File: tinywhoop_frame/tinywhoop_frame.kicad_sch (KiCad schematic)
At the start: 17 parts, among them J1 ESP_conn1, J2 ESP_conn2, J3 ESP_Unused_Pins1, J5 Batt_conn, J6 Conn_02x03_Counter_Clockwise, Q1 2N7002, Q2 2N7002, Q3 2N7002, Q4 2N7002

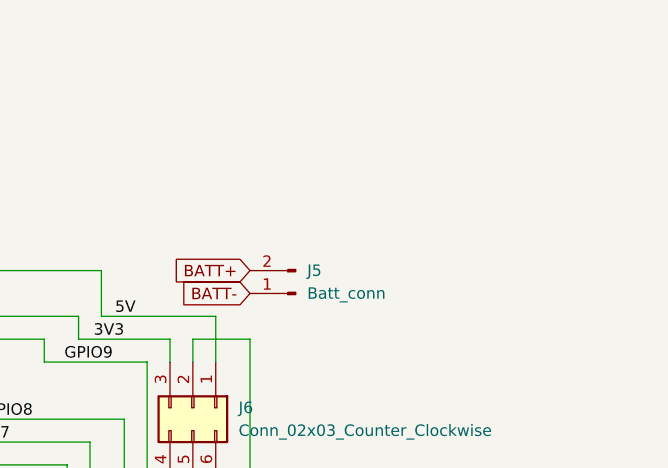
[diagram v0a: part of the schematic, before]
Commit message: pcb updates
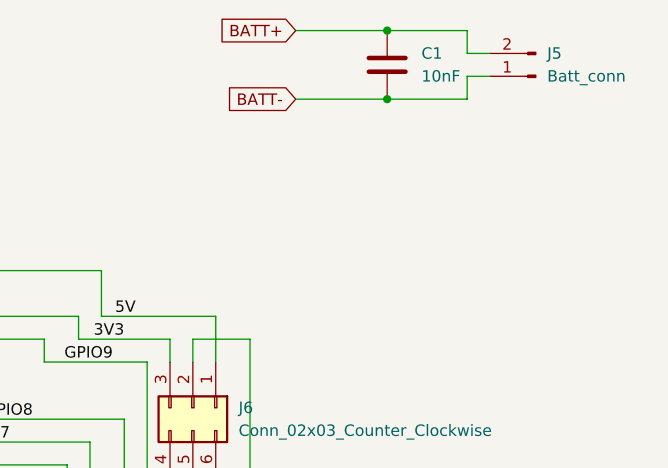
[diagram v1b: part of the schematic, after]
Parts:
- added C1: 10nF, Capacitor_SMD:C_0805_2012Metric_Pad1.18x1.45mm_HandSolder, symbol Device:C
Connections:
- net BATT+: now also C1.1
- net BATT-: now also C1.2
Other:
- moved on the sheet: J5
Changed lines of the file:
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@@
+	)
+	(junction
+		(at 241.3 21.59)
+		(diameter 0)
+		(color 0 0 0 0)
 	)
 	(junction
@@
 	)
 	(junction
+		(at 241.3 29.21)
+		(diameter 0)
+		(color 0 0 0 0)
+	)
+	(junction
 		(at 57.15 53.34)
 		(diameter 0)
@@
 	(wire
 		(pts
+			(xy 250.19 21.59) (xy 241.3 21.59)
+		)
+		(stroke
+			(width 0)
+			(type default)
+		)
+	)
+	(wire
+		(pts
 			(xy 171.45 67.31) (xy 173.99 67.31)
 		)
@@
 	(wire
 		(pts
+			(xy 250.19 26.67) (xy 252.73 26.67)
+		)
+		(stroke
+			(width 0)
+			(type default)
+		)
+	)
+	(wire
+		(pts
 			(xy 97.79 91.44) (xy 105.41 91.44)
 		)
@@
 	(wire
 		(pts
+			(xy 250.19 24.13) (xy 250.19 21.59)
+		)
+		(stroke
+			(width 0)
+			(type default)
+		)
+	)
+	(wire
+		(pts
 			(xy 57.15 96.52) (xy 62.23 96.52)
 		)
@@
 	(wire
 		(pts
+			(xy 231.14 29.21) (xy 241.3 29.21)
+		)
+		(stroke
+			(width 0)
+			(type default)
+		)
+	)
+	(wire
+		(pts
 			(xy 207.01 53.34) (xy 207.01 55.88)
 		)
@@
 	(wire
 		(pts
+			(xy 231.14 21.59) (xy 241.3 21.59)
+		)
+		(stroke
+			(width 0)
+			(type default)
+		)
+	)
+	(wire
+		(pts
 			(xy 219.71 73.66) (xy 219.71 71.12)
 		)
@@
 	(wire
 		(pts
+			(xy 252.73 24.13) (xy 250.19 24.13)
+		)
+		(stroke
+			(width 0)
+			(type default)
+		)
+	)
+	(wire
+		(pts
+			(xy 241.3 29.21) (xy 250.19 29.21)
+		)
+		(stroke
+			(width 0)
+			(type default)
+		)
+	)
+	(wire
+		(pts
 			(xy 187.96 63.5) (xy 187.96 69.85)
 		)
@@
 		(pts
 			(xy 168.91 63.5) (xy 168.91 69.85)
+		)
+		(stroke
+			(width 0)
+			(type default)
+		)
+	)
+	(wire
+		(pts
+			(xy 250.19 29.21) (xy 250.19 26.67)
 		)
 		(stroke
@@
 	(global_label "BATT-"
 		(shape input)
-		(at 226.06 50.8 180)
+		(at 231.14 29.21 180)
 		(fields_autoplaced yes)
 		(effects
@@
 		)
 		(property "Intersheetrefs" "${INTERSHEET_REFS}"
-			(at 217.2086 50.8 0)
+			(at 222.2886 29.21 0)
 			(effects
 				(font
@@
 	(global_label "BATT+"
 		(shape input)
-		(at 226.06 48.26 180)
+		(at 231.14 21.59 180)
 		(fields_autoplaced yes)
 		(effects
@@
 		)
 		(property "Intersheetrefs" "${INTERSHEET_REFS}"
-			(at 217.2086 48.26 0)
+			(at 222.2886 21.59 0)
 			(effects
 				(font
@@
 	(symbol
 		(lib_id "Connector:Conn_01x02_Pin")
-		(at 231.14 50.8 180)
+		(at 257.81 26.67 180)
 		(unit 1)
 		(exclude_from_sim no)
@@
 		(dnp no)
 		(property "Reference" "J5"
-			(at 232.41 48.2599 0)
+			(at 259.08 24.1299 0)
 			(effects
 				(font
@@
 		)
 		(property "Value" "Batt_conn"
-			(at 232.41 50.7999 0)
+			(at 259.08 26.6699 0)
 			(effects
 				(font
@@
 		)
 		(property "Footprint" "Connector_PinHeader_2.54mm:PinHeader_1x02_P2.54mm_Vertical"
-			(at 231.14 50.8 0)
+			(at 257.81 26.67 0)
 			(effects
 				(font
@@
 		)
 		(property "Datasheet" "~"
-			(at 231.14 50.8 0)
+			(at 257.81 26.67 0)
 			(effects
 				(font
@@
 		)
 		(property "Description" "Generic connector, single row, 01x02, script generated"
-			(at 231.14 50.8 0)
+			(at 257.81 26.67 0)
 			(effects
 				(font
@@
 					(unit 1)
 				)
+			)
+		)
+	)
+	(symbol
+		(lib_id "Device:C")
+		(at 241.3 25.4 0)
+		(unit 1)
+		(exclude_from_sim no)
+		(in_bom yes)
+		(on_board yes)
+		(dnp no)
+		(fields_autoplaced yes)
+		(property "Reference" "C1"
+			(at 245.11 24.1299 0)
+			(effects
+				(font
+					(size 1.27 1.27)
+				)
+				(justify left)
+			)
+		)
+		(property "Value" "10nF"
+			(at 245.11 26.6699 0)
+			(effects
+				(font
+					(size 1.27 1.27)
+				)
+				(justify left)
+			)
+		)
+		(property "Footprint" "Capacitor_SMD:C_0805_2012Metric_Pad1.18x1.45mm_HandSolder"
+			(at 242.2652 29.21 0)
+			(effects
+				(font
+					(size 1.27 1.27)
+				)
+				(hide yes)
+			)
+		)
+		(property "Datasheet" "~"
+			(at 241.3 25.4 0)
+			(effects
+				(font
+					(size 1.27 1.27)
+				)
+				(hide yes)
+			)
+		)
+		(property "Description" "Unpolarized capacitor"
+			(at 241.3 25.4 0)
+			(effects
+				(font
+					(size 1.27 1.27)
+				)
+				(hide yes)
+			)
+		)
+		(pin "1"
+		)
+		(pin "2"
+		)
+		(instances
+			(project ""
+				(path "/dcf85f80-a84f-42ea-b7be-95670bbb8f64"
+					(reference "C1")
+					(unit 1)
+				)

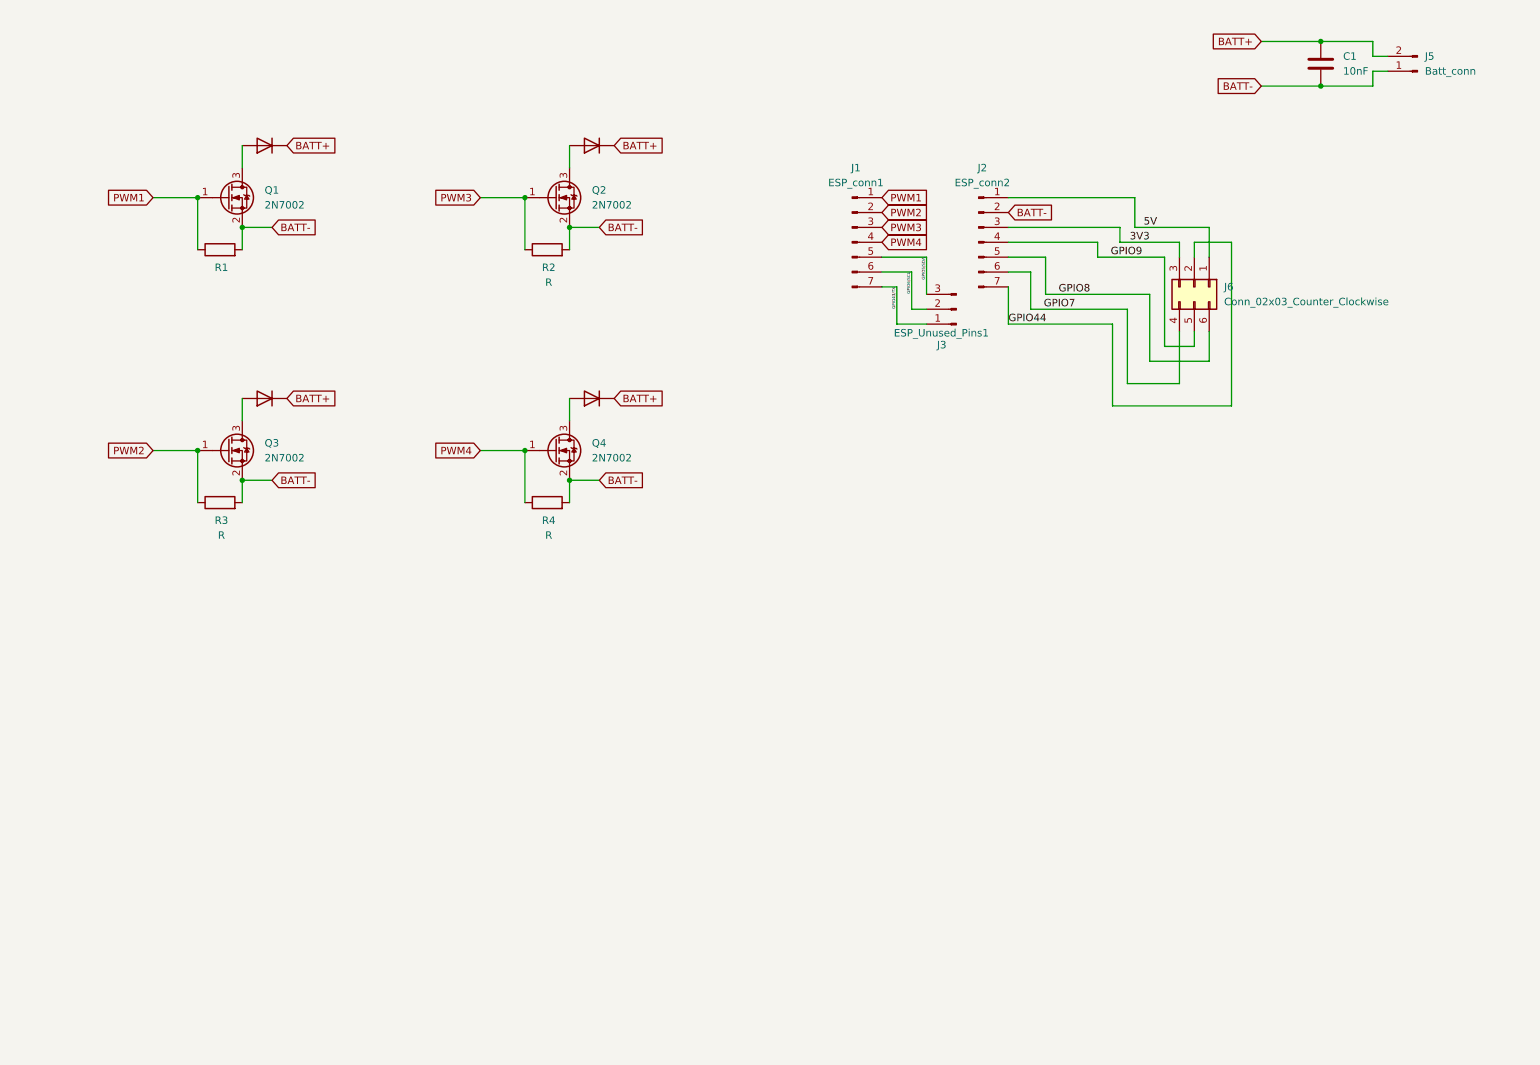
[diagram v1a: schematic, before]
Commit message: updated pcb
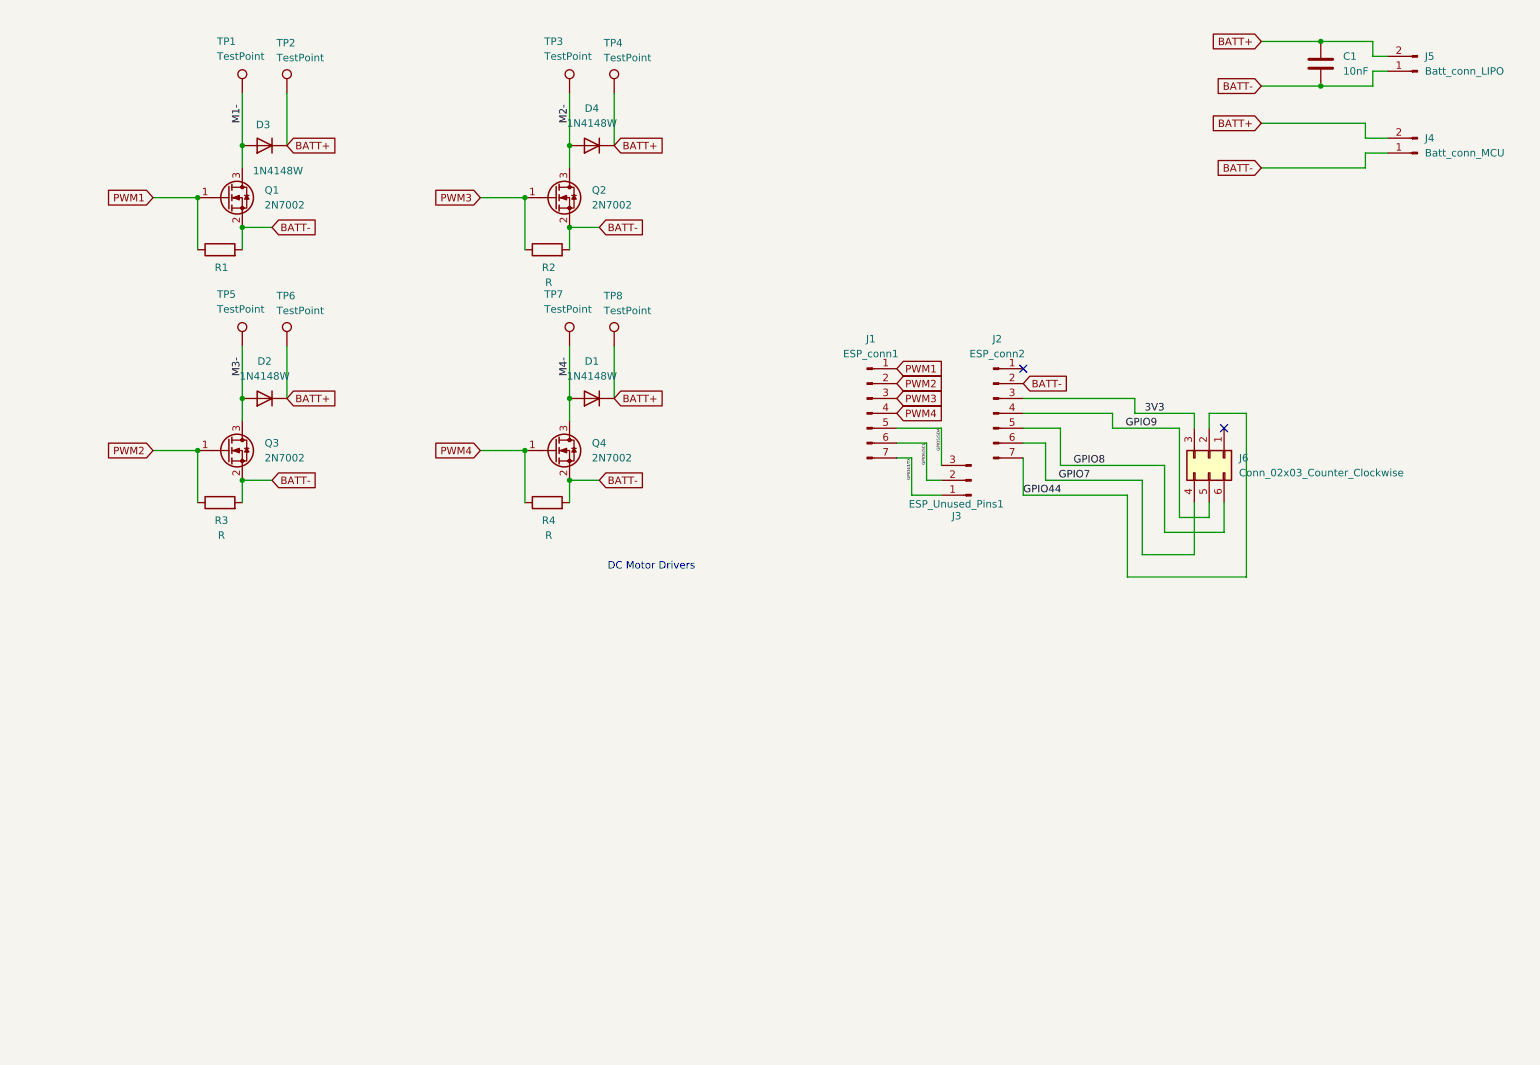
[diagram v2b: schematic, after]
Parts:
- removed D1, D2, D3, D4: D, Diode_THT:D_DO-35_SOD27_P7.62mm_Horizontal, symbol Device:D
- added D1, D2, D3, D4: 1N4148W, Diode_SMD:D_SOD-123, symbol Diode:1N4148W
- added J4: Batt_conn_MCU, Connector_PinHeader_2.54mm:PinHeader_1x02_P2.54mm_Vertical, symbol Connector:Conn_01x02_Pin
- added TP1, TP2, TP3, TP4, TP5, TP6, TP7, TP8: TestPoint, TestPoint:TestPoint_Pad_1.5x1.5mm, symbol Connector:TestPoint
- J5: value Batt_conn -> Batt_conn_LIPO
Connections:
- net BATT+: now also D1.1 (K), D2.1 (K), D3.1 (K), D4.1 (K), J4.2 (Pin_2), TP2.1, TP4.1, TP6.1, TP8.1
- net BATT-: now also J4.1 (Pin_1)
- net M4-: now reaches Q4.3 (D)
- net M4-: now also D1.2 (A), TP7.1
- net M3-: now reaches Q3.3 (D)
- net M3-: now also D2.2 (A), TP5.1
- net M1-: now reaches Q1.3 (D)
- net M1-: now also D3.2 (A), TP1.1
- net M2-: now reaches Q2.3 (D)
- net M2-: now also D4.2 (A), TP3.1
- net 5V: no longer names the net of J6.1 (Pin_1)
- net 5V: no longer J2.1 (Pin_1)
- no-connect marks 0 -> 2
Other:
- note added: "DC Motor Drivers"
- moved on the sheet: J1, J2, J3, J6

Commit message: pcb update
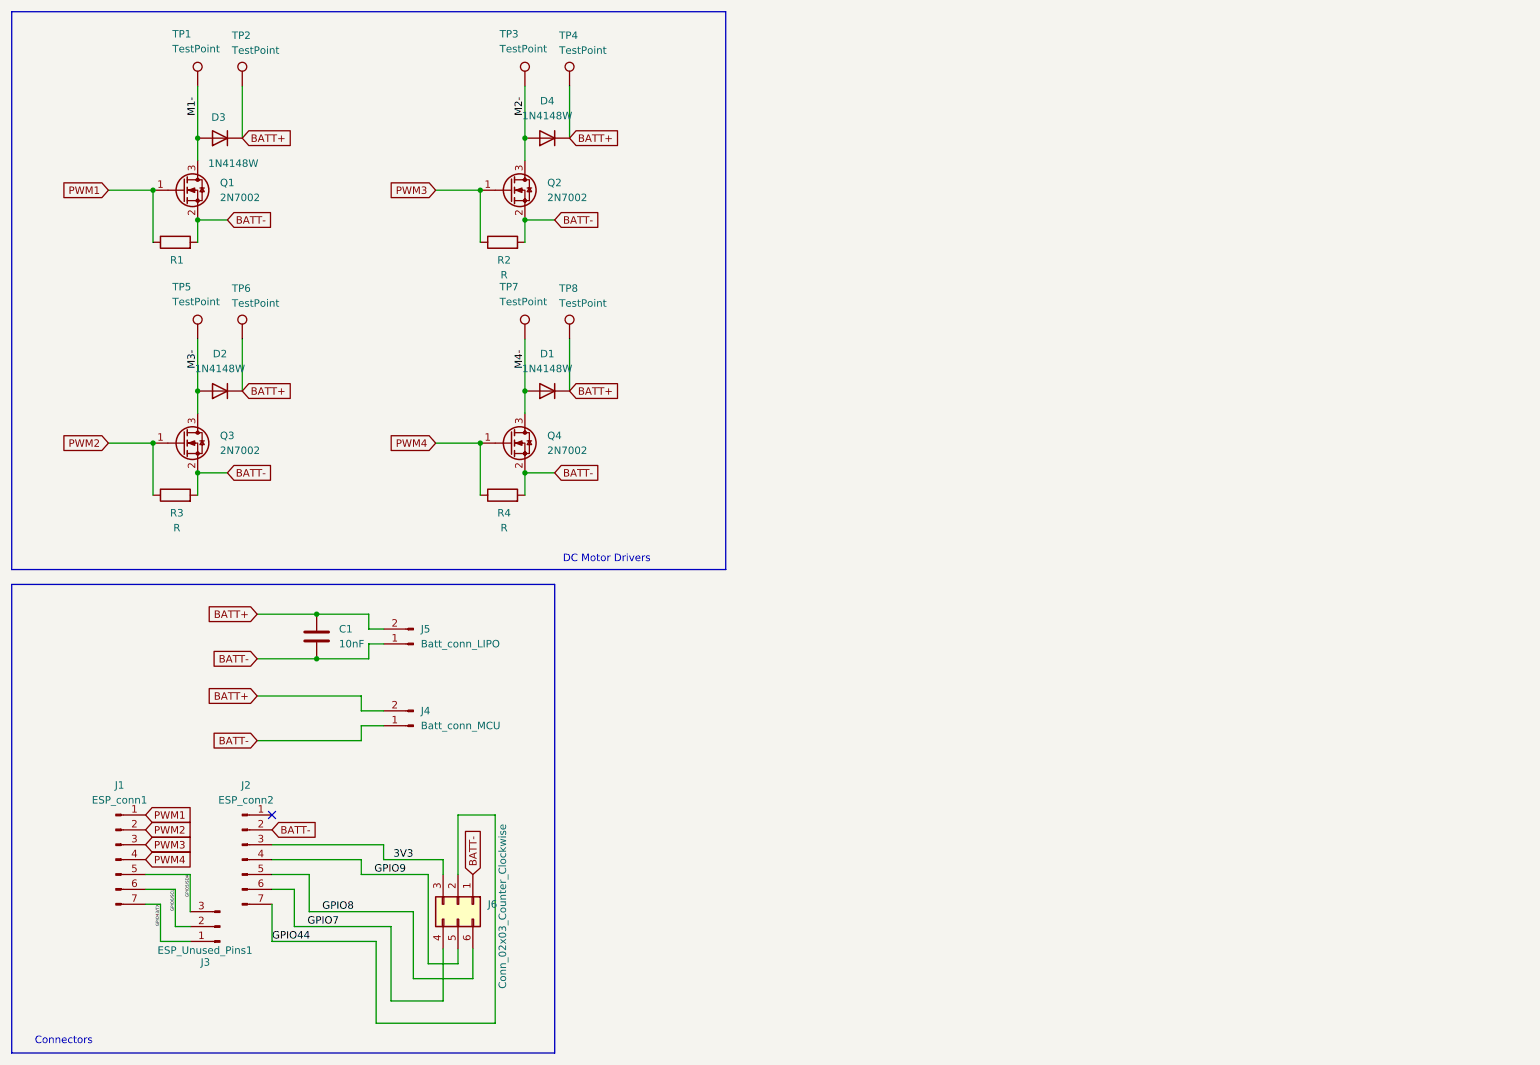
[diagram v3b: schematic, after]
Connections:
- net BATT-: now also J6.1 (Pin_1)
- no-connect marks 2 -> 1
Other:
- note added: "Connectors"
- moved on the sheet: C1, D1, D2, D3, D4, J1, J2, J3, J4, J5, J6, Q1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
